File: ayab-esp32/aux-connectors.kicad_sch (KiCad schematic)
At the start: 31 parts, among them J801 AYAB_UART, J802 I2C_VBUS, J803 USER_I2C, J804 I2C_VBUS, J805 AYAB_SPI, J806 AYAB_I2C, Q801 AO3400A, Q802 AO3400A, Q803 AO3400A, Q804 AO3400A

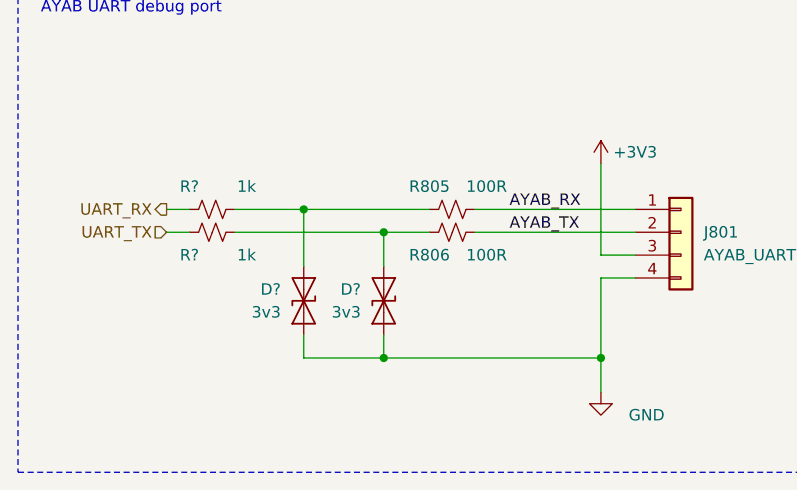
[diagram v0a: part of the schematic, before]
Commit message: production files
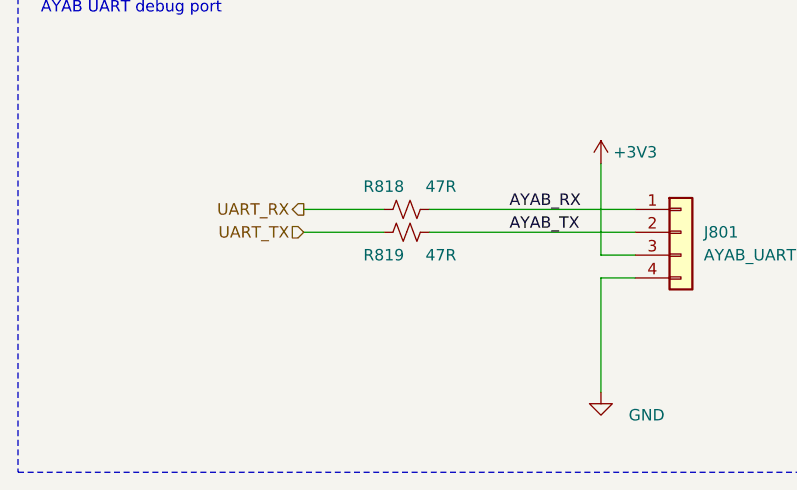
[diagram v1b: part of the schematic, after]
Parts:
- removed D? (x2): 3v3, Diode_SMD:D_SOD-923, symbol Diode:ESD9B3.3ST5G
- removed R805, R806: 100R, Resistor_SMD:R_0603_1608Metric, symbol ayab-lib:R_Small_US
- R818, R819: renamed from R?; value 1k -> 47R
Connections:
- net AYAB_RX: now also R818.2
- net AYAB_TX: now also R819.1
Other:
- moved on the sheet: R818, R819
